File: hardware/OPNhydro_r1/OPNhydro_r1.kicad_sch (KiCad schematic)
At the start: 88 parts, among them J1 JACK_5MM, J11 Float_Low, J12 BME280, J14 Float_High, J15 PH, J3 BH1750, J4 1-Wire, J6 OLED, J7 HC-SR04, Q1 2N7002K, Q2 AO3400A, Q3 AO3400A, Q4 AO3400A, Q5 AO3400A, Q8 AO3400A, U1 SI2301, U2 TPS62933, U3 ADM3260

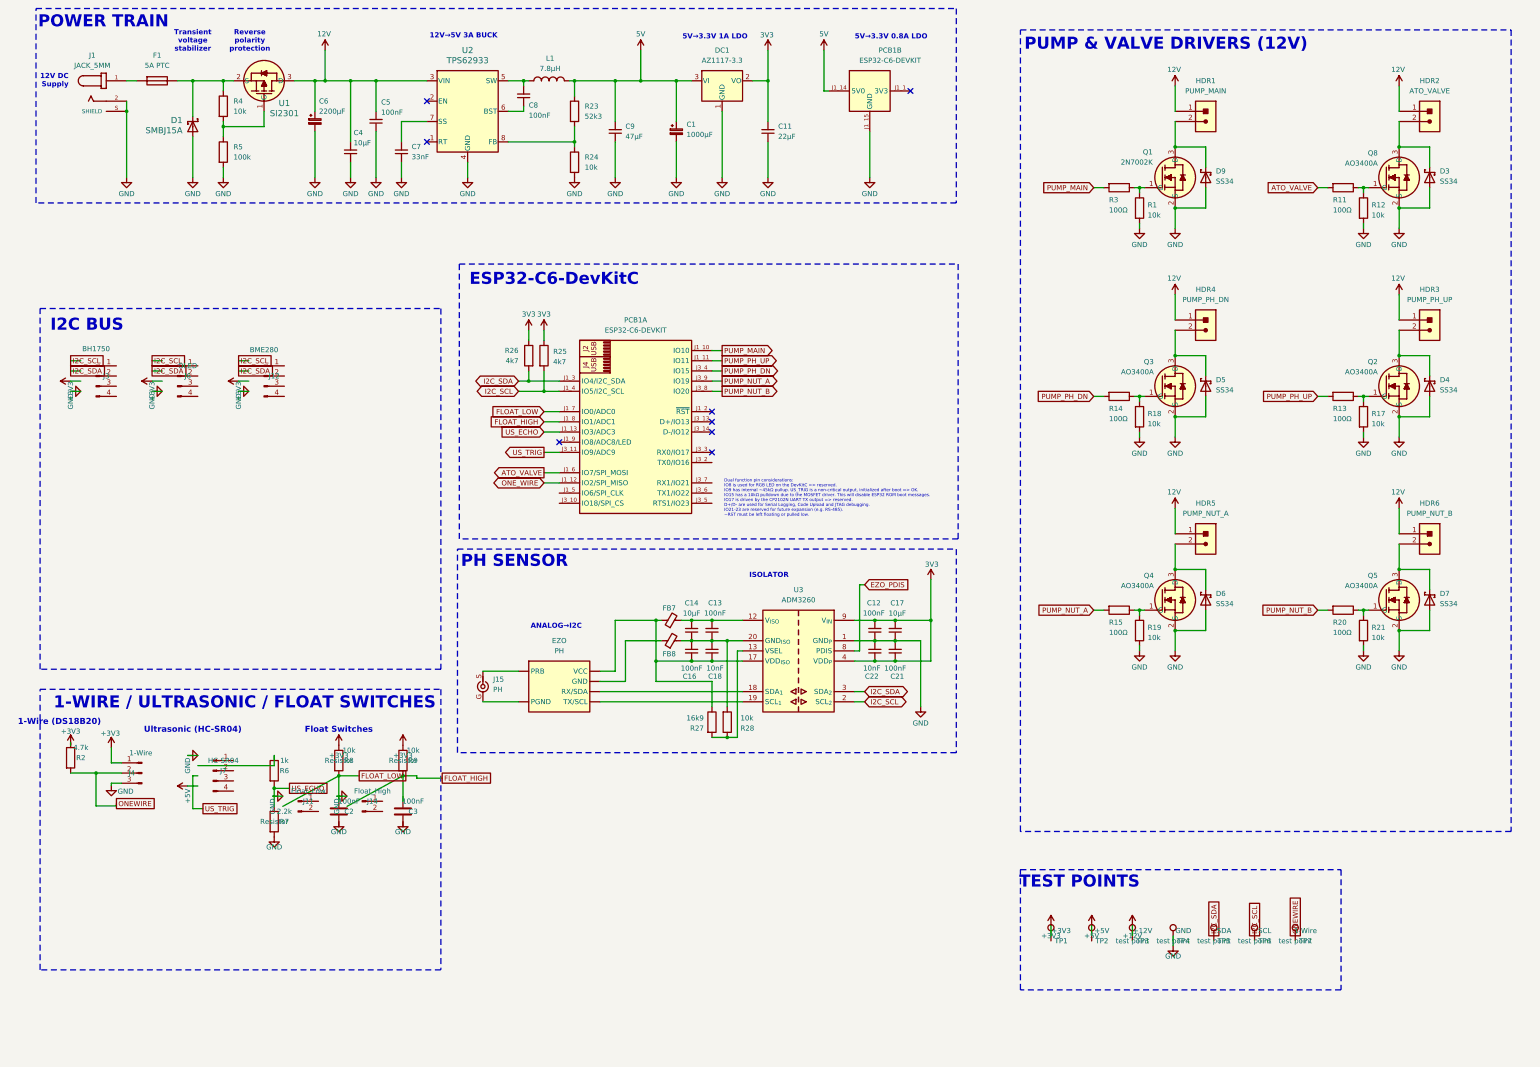
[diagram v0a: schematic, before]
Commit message: update w design and schematic
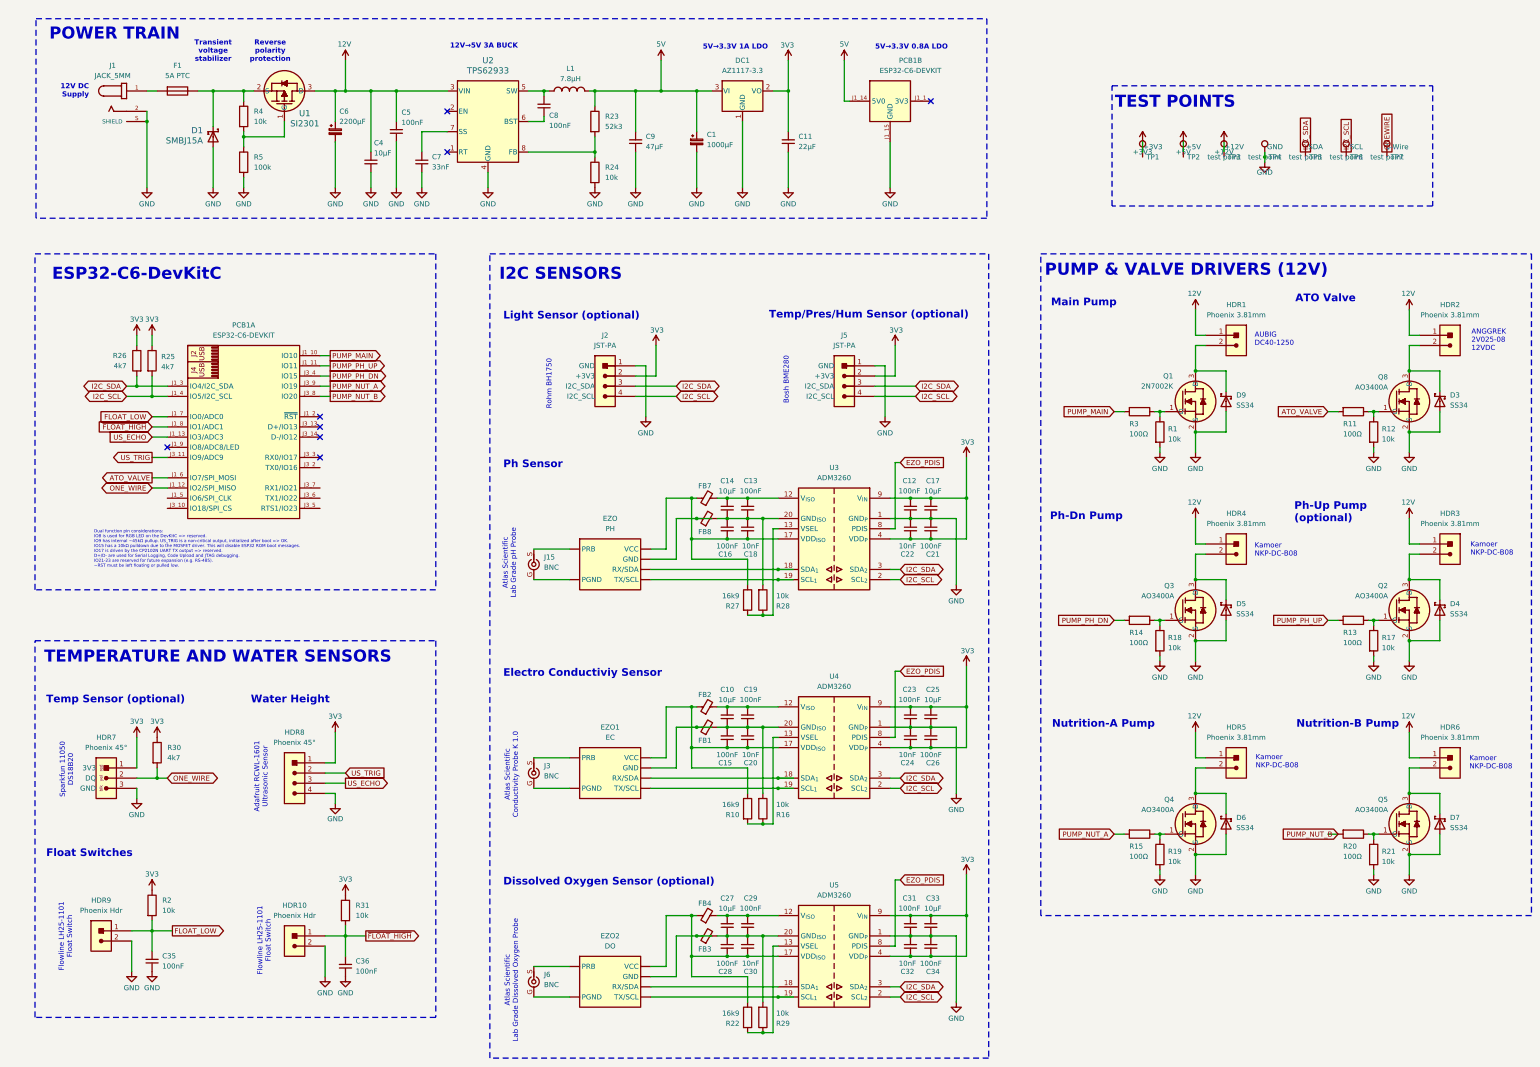
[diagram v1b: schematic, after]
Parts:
- removed C2, C3: 100nF, Capacitor_SMD:C_0805_2012Metric, symbol Device:C
- removed J11: Float_Low, Connector_JST:JST_XH_B2B-XH-A_1x02_P2.50mm_Vertical, symbol Connector:Conn_01x02_Pin
- removed J12: BME280, Connector_JST:JST_PH_B4B-PH-K_1x04_P2.00mm_Vertical, symbol Connector:Conn_01x04_Pin
- removed J14: Float_High, Connector_JST:JST_XH_B2B-XH-A_1x02_P2.50mm_Vertical, symbol Connector:Conn_01x02_Pin
- removed J3: BH1750, Connector_JST:JST_PH_B4B-PH-K_1x04_P2.00mm_Vertical, symbol Connector:Conn_01x04_Pin
- removed J4: 1-Wire, Connector_JST:JST_PH_B3B-PH-K_1x03_P2.00mm_Vertical, symbol Connector:Conn_01x03_Pin
- removed J6: OLED, Connector_JST:JST_PH_B4B-PH-K_1x04_P2.00mm_Vertical, symbol Connector:Conn_01x04_Pin
- removed J7: HC-SR04, Connector_JST:JST_XH_B4B-XH-A_1x04_P2.50mm_Vertical, symbol Connector:Conn_01x04_Pin
- removed R2: 4.7k, Resistor_SMD:R_0805_2012Metric, symbol Device:R
- removed R6: 1k, Resistor_SMD:R_0805_2012Metric, symbol Device:R
- removed R7: 2.2k, Resistor_SMD:R_0805_2012Metric, symbol Device:R
- removed R8, R9: 10k, Resistor_SMD:R_0805_2012Metric, symbol Device:R
- added C10, C25, C27, C33: 10μF, Coert-Vonk:CAP X7R 10μF ±10 16V 0805, symbol Coert-Vonk:CAP X7R 10μF ±10% 16V 0805
- added C15, C19, C23, C26, C28, C29, C31, C34, C35, C36: 100nF, Coert-Vonk:CAP X7R 100nF ±10 25V 0805, symbol Coert-Vonk:CAP X7R 100nF ±10% 25V 0805
- added C20, C24, C30, C32: 10nF, Coert-Vonk:CAP X7R 10nF ±10% 50V 0805, symbol Coert-Vonk:CAP X7R 10nF ±10% 50V 0805
- added EZO1: EC, symbol Coert-Vonk:EVAL EZO pH
- added EZO2: DO, symbol Coert-Vonk:EVAL EZO pH
- added FB1, FB2, FB3, FB4: 330Ω at 100MHz, Coert-Vonk:FERRITE BEAD 330Ω 0805, symbol Coert-Vonk:FERRITE BEAD 330Ω 0805
- added HDR10, HDR9: Phoenix Hdr, Coert-Vonk:TERM BLOCK HDR 2POS RA 3.81mm 1803277, symbol Coert-Vonk:TERM BLOCK HDR 2POS RA 3.81mm
- added HDR7: Phoenix 45°, Coert-Vonk:TERM BLOCK HDR 1WIRE 3POS RA 3.81mm 1803280, symbol Coert-Vonk:TERM BLOCK HDR 3POS 1WIRE RA 3.81mm
- added HDR8: Phoenix 45°, Coert-Vonk:TERM BLOCK HDR 1WIRE 3POS RA 3.81mm 1803280, symbol Coert-Vonk:TERM BLOCK HDR 4POS RA 3.81mm
- added J2, J5: JST-PA, Coert-Vonk:CONN MALE 4POS RA 2mm I2C JST S04B-PASK-2, symbol Coert-Vonk:CONN I2C MALE 4POS RA 2mm JST S04B-PASK-2
- added J3, J6: BNC, Coert-Vonk:CONN BNC JACK RA 50Ω, symbol Coert-Vonk:CONN BNC JACK RA 50Ω 5227161-6
- added R10, R22: 16k9, Coert-Vonk:RES 16.9kΩ ±1 18W 0805, symbol Coert-Vonk:RES 16.9kΩ ±1% 1/8W 0805
- added R16, R29: 10k, Coert-Vonk:RES 10kΩ 0805, symbol Coert-Vonk:RES 10kΩ ±1% 1/8W 0805
- added R2, R31: 10k, Coert-Vonk:RES 10kΩ ±1 18W Yageo 0805, symbol Coert-Vonk:RES 10kΩ ±1% 1/8W Yageo 0805
- added R30: 4k7, Coert-Vonk:RES 4.7kΩ ±1 18W Yageo 0805, symbol Coert-Vonk:RES 4.7kΩ ±1% 1/8W Yageo 0805
- added U4, U5: ADM3260, Coert-Vonk:IC ISOLTR 2.5KV 2CH I2C 20SSOP ADM3260, symbol Coert-Vonk:IC ISOLTR 2.5KV 2CH I2C 20SSOP ADM3260
- HDR1: value PUMP_MAIN -> Phoenix 3.81mm
- HDR2: value ATO_VALVE -> Phoenix 3.81mm
- HDR3: value PUMP_PH_UP -> Phoenix 3.81mm
- HDR4: value PUMP_PH_DN -> Phoenix 3.81mm
- HDR5: value PUMP_NUT_A -> Phoenix 3.81mm
- HDR6: value PUMP_NUT_B -> Phoenix 3.81mm
- J15: value PH -> BNC
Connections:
- net 3V3: now also C23.2, C24.2, C25.2, C26.2, C31.2, C32.2, C33.2, C34.2, HDR7.1 (3V3), HDR8.1, J2.2 (+3V3), J5.2 (+3V3), R2.2, R30.2, R31.2, U4.4 (VDD_{P}), U4.9 (V_{IN}), U5.4 (VDD_{P}), U5.9 (V_{IN})
- net EZO_PDIS: now also U4.8 (PDIS), U5.8 (PDIS)
- net FLOAT_LOW: now also C35.2, HDR9.1, R2.1
- net GND: now also TP4.1, C23.1, C24.1, C25.1, C26.1, C31.1, C32.1, C33.1, C34.1, C35.1, C36.1, HDR10.2, HDR7.3 (GND), HDR8.4, HDR9.2, J2.1 (GND), J5.1 (GND), U4.1 (GND_{P}), U4.10 (GND_{P}), U4.5 (GND_{P}), U4.7 (GND_{P}), U5.1 (GND_{P}), U5.10 (GND_{P}), U5.5 (GND_{P}), U5.7 (GND_{P})
- net I2C_SCL: now also J2.4 (I2C_SCL), J5.4 (I2C_SCL), U4.2 (SCL_{2}), U5.2 (SCL_{2})
- net I2C_SDA: now also J2.3 (I2C_SDA), J5.3 (I2C_SDA), U4.3 (SDA_{2}), U5.3 (SDA_{2})
- net ONE_WIRE: now also HDR7.2 (DQ), R30.1
- net US_ECHO: now also HDR8.3
- net US_TRIG: now also HDR8.2
- net FLOAT_HIGH renamed ~{FLOAT_HIGH}
- net ~{FLOAT_HIGH}: now also C36.2, HDR10.1, R31.1
- new net: C15.2, C20.2, EZO1.6 (VCC), FB1.1, R10.2, U4.17 (VDD_{ISO})
- new net: C10.2, C19.2, FB1.2, U4.12 (V_{ISO})
- new net: C10.1, C15.1, C19.1, C20.1, FB2.2, R16.1, U4.11 (GND_{ISO}), U4.14 (GND_{ISO}), U4.16 (GND_{ISO}), U4.20 (GND_{ISO})
- new net: R10.1, R16.2, U4.13 (VSEL)
- new net: EZO1.3 (RX/SDA), U4.18 (SDA_{1})
- new net: EZO1.2 (TX/SCL), U4.19 (SCL_{1})
- new net: C27.1, C28.1, C29.1, C30.1, FB4.2, R29.1, U5.11 (GND_{ISO}), U5.14 (GND_{ISO}), U5.16 (GND_{ISO}), U5.20 (GND_{ISO})
- new net: R22.1, R29.2, U5.13 (VSEL)
- new net: C27.2, C29.2, FB3.2, U5.12 (V_{ISO})
- new net: EZO2.1 (GND), FB4.1
- new net: EZO2.2 (TX/SCL), U5.19 (SCL_{1})
- new net: EZO2.3 (RX/SDA), U5.18 (SDA_{1})
- new net: EZO2.4 (PGND), J6.G (GND)
- new net: EZO2.5 (PRB), J6.S
- new net: C28.2, C30.2, EZO2.6 (VCC), FB3.1, R22.2, U5.17 (VDD_{ISO})
- new net: EZO1.1 (GND), FB2.1
- new net: EZO1.4 (PGND), J3.G (GND)
- new net: EZO1.5 (PRB), J3.S
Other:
- note added: "ANGGREK 2V025-08 12VDC"
- note added: "ATO Valve"
- note added: "AUBIG DC40-1250"
- note added: "Adafruit RCWL-1601 Ultrasonic Sensor"
- note added: "Atlas Scientific Conductivity Probe K 1.0"
- note added: "Atlas Scientific Lab Grade Dissolved Oxygen Probe"
- note added: "Atlas Scientific Lab Grade pH Probe"
- note added: "Bosh BME280"
- note added: "Dissolved Oxygen Sensor (optional)"
- note added: "Electro Conductiviy Sensor"
- note added: "Flowline LH25-1101 Float Switch"
- note added: "I2C SENSORS"
- note added: "Kamoer NKP-DC-B08"
- note added: "Light Sensor (optional)"
- note added: "Main Pump"
- note added: "Nutrition-A Pump"
- note added: "Nutrition-B Pump"
- note added: "Ph Sensor"
- note added: "Ph-Dn Pump"
- note added: "Ph-Up Pump (optional)"
- note added: "Rohm BH1750"
- note added: "Sparkfun 11050 DS18B20"
- note added: "TEMPERATURE AND WATER SENSORS"
- note added: "Temp Sensor (optional)"
- note added: "Temp/Pres/Hum Sensor (optional)"
- note added: "Water Height"
- note removed: "1-WIRE / ULTRASONIC / FLOAT SWITCHES"
- note removed: "1-Wire (DS18B20)"
- note removed: "ANALOG→I2C"
- note removed: "I2C BUS"
- note removed: "ISOLATOR"
- note removed: "PH SENSOR"
- note removed: "Ultrasonic (HC-SR04)"
- moved on the sheet: C1, C11, C12, C13, C14, C16, C17, C18, C21, C22, C4, C5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
